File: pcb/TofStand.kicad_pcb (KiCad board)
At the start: 2 copper layers, 87 x 88 mm, 187 parts, among them Q1 BC848, Q10 BC848, Q11 BC848, Q14 MMBT2222, Q2 BC848, Q5 DVIUC6-4SC6, Q6 BC848, Q7 BC848, SW1 DIPx4, SW2 SWITCH_H, SW3 BUTTON, SW4 SWITCH_2x, SW5 SWITCH_2x, U1 L6470, U2 L6470

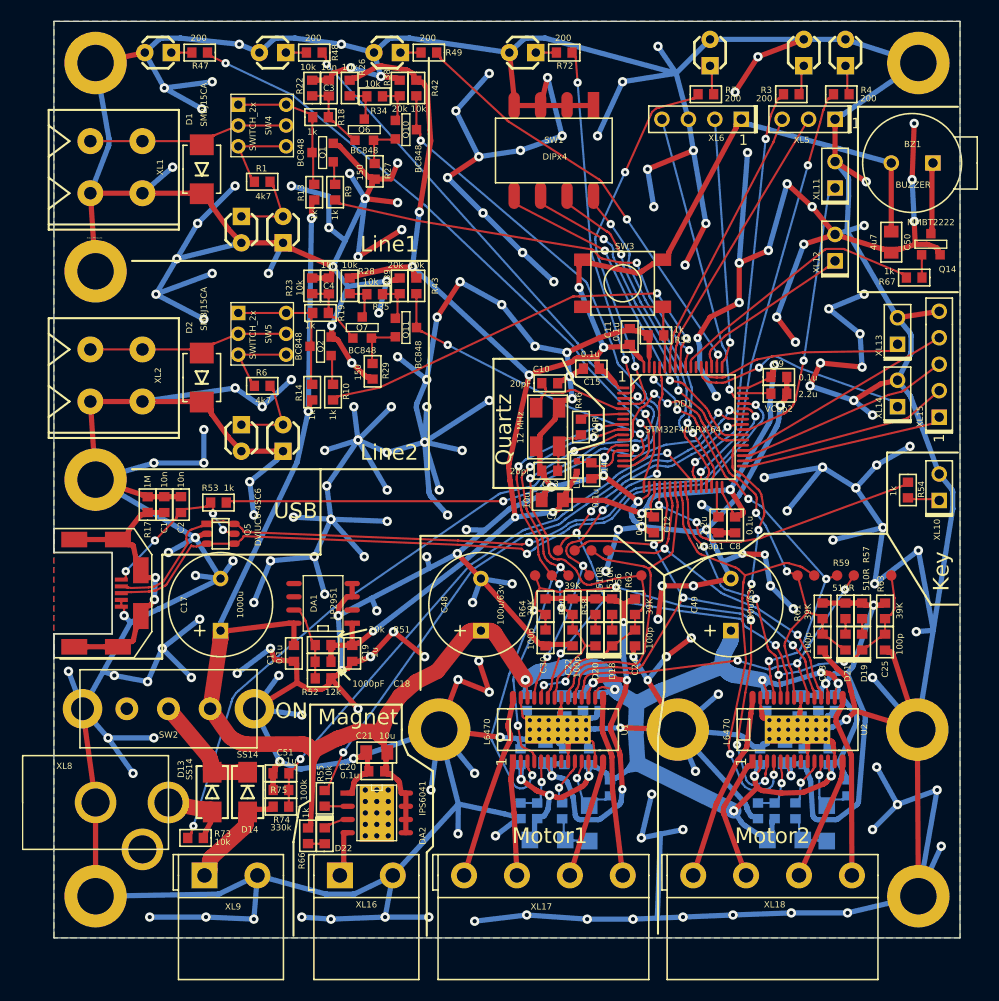
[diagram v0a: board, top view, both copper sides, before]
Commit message: PCB sent to factory
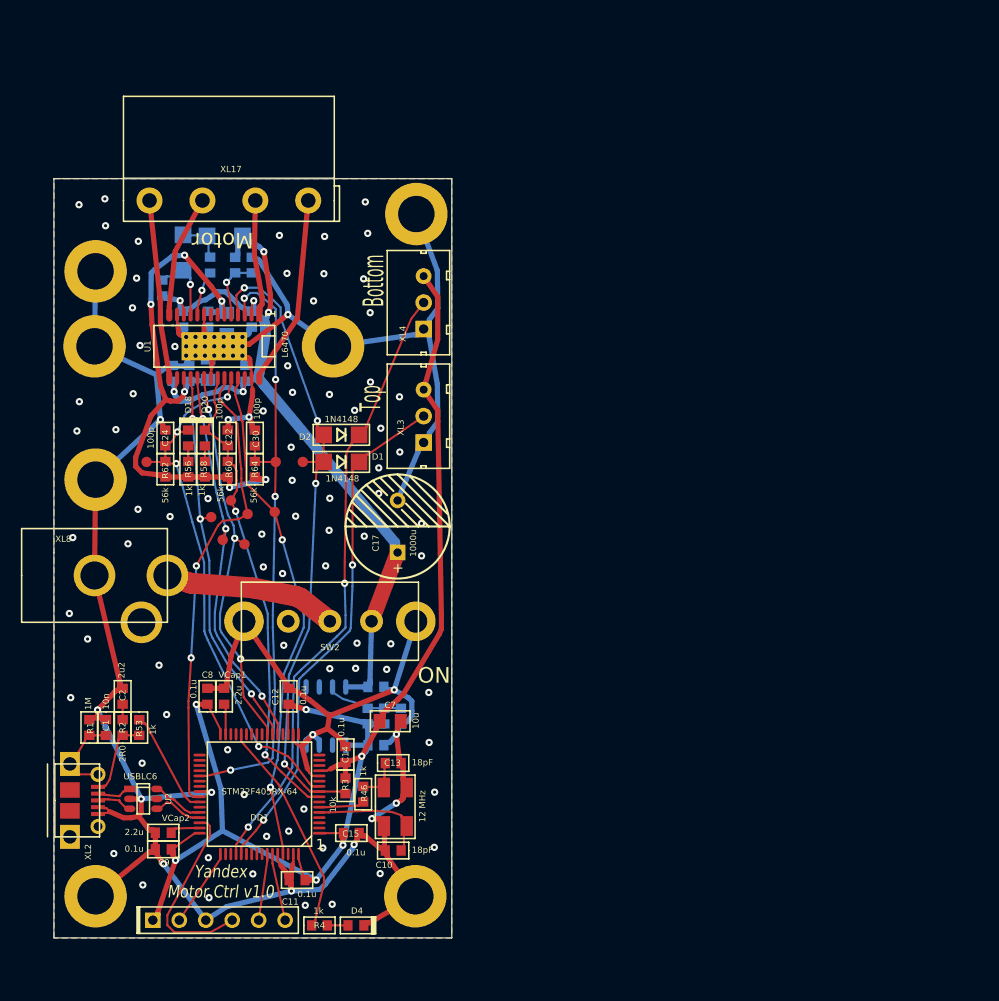
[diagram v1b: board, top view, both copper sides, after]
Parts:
- removed BZ1: BUZZER, Installation:BUZZER_HC0903
- removed C20, C28, C29, C51: 0.1u, Capacitors:CAP_0603
- removed C21, C34: 10u, Capacitors:CAP_0805
- removed C23, C25: 100p, Capacitors:CAP_0603
- removed C3, C4: 10n, Capacitors:CAP_0603
- removed C35: 4u7/63v, Capacitors:CAP_0805
- removed C38: 220n/16v, Capacitors:CAP_0603
- removed C39: 10n/50v, Capacitors:CAP_0603
- removed C41, C43, C45, C47: 0.1u/50v, Capacitors:CAP_0603
- removed C48, C49: 100u/63v, Capacitors:CAP_10xxR
- removed C50: 4u7, Capacitors:CAP_0805
- removed D10, D15, D16, D17, D27, D3, D5, D6, D7, D9: LED, LEDs:LED_Through-Hole-3mm
- removed D13, D14: SS14, Diodes:SMA_DO214AC
- removed D19, D21, D22: LED, LEDs:LED_0603
- removed D24, D26: 1N4148, Diodes:SOD80C
- removed DA2: IPS6041, SO_DIL_TSSOP:SO8HEATSINK
- removed HOLE3, HOLE9: HOLE_METALLED, PCB:Hole3_5_out6mm
- removed L1: BLM, Inductors:IND_0402
- removed Q1, Q10, Q11, Q2, Q6, Q7: BC848, SOT:SOT23-3
- removed Q14: MMBT2222, SOT:SOT23-3
- removed Q5: DVIUC6-4SC6, SOT:SOT23-6
- removed R10, R13, R14, R18, R19, R50, R54, R66, R67, R9: 1k, Resistors:RES_0603
- removed R17: 1M, Resistors:RES_0603
- removed R22, R23, R26, R28, R34, R35, R42, R43, R55, R73: 10k, Resistors:RES_0603
- removed R27, R29: 150, Resistors:RES_0603
- removed R38, R39: 20k, Resistors:RES_0603
- removed R47, R48, R49, R7, R72: 200, Resistors:RES_0603
- removed R57, R59: 510R, Resistors:RES_0603
- removed R6, R71: 4k7, Resistors:RES_0603
- removed R61, R63: 39K, Resistors:RES_0603
- removed R70: 33k, Resistors:RES_0603
- removed R74: 330k, Resistors:RES_0603
- removed R75: 100k, Resistors:RES_0603
- removed SW1: DIPx4, BtnsSwitches:DIP_SMD_X4
- removed SW3: BUTTON, BtnsSwitches:BTN_6x6
- removed SW4, SW5: SWITCH_2x, BtnsSwitches:BTN_PSM6
- removed TP10, TP11, TP12, TP13, TP14: TESTPOINT, PCB:TESTPOINT_1MM
- removed XL10, XL11, XL12, XL13, XL14: CONN_2, Connectors:PLS-2
- removed XL15: CONN_5, Connectors:PLS-5
- removed XL16, XL9: CONN_2, Connectors:TermiBlockHeader_508_x2_R
- removed XL18: CONN_4, Connectors:TermiBlockHeader_508_x4_R
- removed XL5: CONN_3, Connectors:PLS-3
- removed XL6: ST_SWD, Connectors:PLS-4
- removed XL7: USB_MICRO_B, Connectors:USBmicro_MOLEX_WM17142
- added R2: 2R0, Resistors:RES_0603, F.Cu at (74.6, 95.8)
- added XL3: CONN_3, Connectors:W03_Pitch_2d54, F.Cu at (103.5, 65.9)
- added XL4: CONN_3, Connectors:W03_Pitch_2d54, F.Cu at (103.5, 55.0)
- C10, C13: value 20pF -> 18pF
- C16, C18, C19, R51, R52: moved to B.Cu
- C2: value 10n -> 2u2
- C33: value 4u7/63v -> 10u
- C36: value 220n/16v -> 220n
- C37: value 10n/50v -> 10n
- C40, C42, C44, C46: value 0.1u/50v -> 0.1u
- D1, D2: value SMBJ15CA -> 1N4148; footprint Diodes:SMB_DO214AA -> Diodes:SOD80C
- D4: footprint LEDs:LED_Through-Hole-3mm -> LEDs:LED_0603
- DA1: footprint SO_DIL_TSSOP:SO8 -> SO_DIL_TSSOP:SO8_150MIL; moved to B.Cu
- R1: value 4k7 -> 1M
- R3: value 200 -> 10k
- R4: value 200 -> 1k
- R46: value 200R -> 1k
- R56, R58: value 510R -> 1k
- R60, R62, R64: value 39K -> 56k
- U2: value L6470 -> USBLC6; footprint SO_DIL_TSSOP:HTSSOP28 -> SOT:SOT23-6
- XL1: value CONN_2 -> CONN_6; footprint Connectors:SPRING_TERM_XY124V_A_2 -> Connectors:PLS-6
- XL2: value CONN_2 -> USB_MICRO; footprint Connectors:SPRING_TERM_XY124V_A_2 -> Connectors:USBmicro_MOLEX_1050170001
- moved D4 96.1 mm to (97.0, 114.8), turned to 0 degrees
- moved R4 94.2 mm to (93.5, 114.8)
- moved R3 79.0 mm to (96.0, 101.4), turned to 270 degrees
- moved C9 74.5 mm to (78.5, 107.5), turned to 180 degrees
- moved VCap2 72.6 mm to (78.5, 105.9), turned to 180 degrees
- moved XL1 72.4 mm to (77.5, 114.3), turned to 0 degrees
- moved XL17 71.5 mm to (84.8, 45.2), turned to 180 degrees
- moved D23 67.3 mm to (80.4, 50.2), turned to 90 degrees
- moved HOLE10 67.0 mm to (71.9, 59.2), turned to 180 degrees
- moved D25 65.8 mm to (84.4, 48.6), turned to 0 degrees
- moved C36 64.4 mm to (78.4, 53.6), turned to 270 degrees
- moved U2 63.2 mm to (76.6, 102.6)
- moved C37 62.4 mm to (83.0, 51.4), turned to 270 degrees
- moved TP6 62.1 mm to (86.6, 75.3)
- moved TP9 62.0 mm to (83.1, 75.6)
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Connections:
- net /LED_BT_LOW renamed Net-(DD1-Pad28)
- C1 pad 1: /SHLD -> GND
- C1 pad 2: GND -> Net-(C1-Pad2)
- C11 pad 1: +3.3V -> +3v3
- C12 pad 1: +3.3V -> +3v3
- C14 pad 1: Net-(C14-Pad1) -> +3v3
- C15 pad 1: +3.3V -> +3v3
- C16 pad 1: +12V -> +12v
- C17 pad 1: +12V -> +12v
- C18 pad 1: +3.3V -> +3v3
- C19 pad 1: +3.3V -> +3v3
- C2 pad 1: GND -> Net-(C2-Pad1)
- C2 pad 2: /5V_USB -> GND
- C36 pad 2: +12V -> +12v
- C40 pad 1: +12V -> +12v
- C42 pad 1: +12V -> +12v
- C44 pad 1: +12V -> +12v
- C46 pad 1: +12V -> +12v
- C7 pad 1: +3.3V -> +3v3
- C8 pad 1: +3.3V -> +3v3
- C9 pad 1: +3.3V -> +3v3
- D1 pad A: /LineIn1 -> /SW_1
- D1 pad C: GND -> /ENDSTOP_TOP
- D2 pad A: /LineIn2 -> /SW_1
- D2 pad C: GND -> /ENDSTOP_BOT
- D25 pad A: +12V -> +12v
- DA1 pad 1: +3.3V -> +3v3
- DA1 pad 8: +12V -> +12v
- DD1 pad 1: +3.3V -> +3v3
- DD1 pad 11: /BUSY/SYNC_2 -> (no net)
- DD1 pad 13: Net-(C14-Pad1) -> +3v3
- DD1 pad 14: /TrgOut1 -> (no net)
- DD1 pad 15: /TrgOut2 -> (no net)
- DD1 pad 16: /LED1 -> (no net)
- DD1 pad 17: /LED2 -> (no net)
- DD1 pad 19: +3.3V -> +3v3
- DD1 pad 2: /LED4 -> (no net)
- DD1 pad 20: Net-(DD1-Pad20) -> (no net)
- DD1 pad 24: /SW_2 -> (no net)
- DD1 pad 25: /FLAG_2 -> (no net)
- DD1 pad 26: /BatteryMeas -> (no net)
- DD1 pad 27: /LED_BT_PWR -> (no net)
- DD1 pad 29: /DS1 -> (no net)
- DD1 pad 3: /PwrSrcSns -> (no net)
- DD1 pad 30: /DS2 -> (no net)
- DD1 pad 32: +3.3V -> +3v3
- DD1 pad 33: /RSL1 -> (no net)
- DD1 pad 34: /RSL2 -> (no net)
- DD1 pad 35: /RSL3 -> (no net)
- DD1 pad 36: /RSL4 -> (no net)
- DD1 pad 38: /DS3 -> (no net)
- DD1 pad 39: /DS4 -> (no net)
- DD1 pad 4: /LED_SRC_PWR -> (no net)
- DD1 pad 40: /GPIO1 -> GND
- DD1 pad 43: /MagnetIN -> (no net)
- DD1 pad 44: /D- -> /USB_D-
- DD1 pad 45: /D+ -> /USB_D+
- DD1 pad 48: +3.3V -> +3v3
- DD1 pad 50: /LED3 -> (no net)
- DD1 pad 51: /GPIO2 -> (no net)
- DD1 pad 52: /GPIO3 -> /ENDSTOP_BOT
- DD1 pad 53: /GPIO4 -> /ENDSTOP_TOP
- DD1 pad 55: /Buzzer -> (no net)
- DD1 pad 56: /LineTx1 -> (no net)
- DD1 pad 57: /LineTx2 -> (no net)
- DD1 pad 58: /DBG_UART_TX -> /UART_TX
- DD1 pad 59: /DBG_UART_RX -> /UART_RX
- DD1 pad 60: Net-(DD1-Pad60) -> GND
- DD1 pad 62: /STEP_CLK_2 -> (no net)
- DD1 pad 64: +3.3V -> +3v3
- R1 pad 1: Net-(R1-Pad1) -> Net-(C1-Pad2)
- R1 pad 2: Net-(D5-PadA) -> GND
- R3 pad 1: /LED_BT_PWR -> +3v3
- R3 pad 2: Net-(D3-PadA) -> /SW_1
- R51 pad 1: +3.3V -> +3v3
- R68 pad 1: +12V -> +12v
- SW2 pad 1: +12V -> +12v
- TP4 pad 1: /BUSY/SYNC_2 -> /STEP_CLK_1
- TP5 pad 1: /SW_2 -> /STBY/RST
- TP6 pad 1: /FLAG_2 -> /MOTOR_CS
- TP7 pad 1: /STEP_CLK_1 -> /MOTOR_SCK
- TP8 pad 1: /STEP_CLK_2 -> /MOTOR_MOSI
- TP9 pad 1: /SDI_2 -> /MOTOR_MISO
- U1 pad 12: +12V -> +12v
- U1 pad 16: +12V -> +12v
- U1 pad 18: /SDI_2 -> /MOTOR_MISO
- U1 pad 2: +12V -> +12v
- U1 pad 26: +12V -> +12v
- U2 pad 1: /OUT2_1A -> /DIN-
- U2 pad 2: +12V -> GND
- U2 pad 3: /STBY/RST -> /DIN+
- U2 pad 4: /SW_2 -> /USB_D+
- U2 pad 5: /ADC_2 -> (no net)
- U2 pad 6: /Vdd2 -> /USB_D-
- XL1 pad 1: /LineIn1 -> +3v3
- XL1 pad 2: GND -> /SWCLK
- XL2 pad 1: /LineIn2 -> /5V_USB
- XL2 pad 2: GND -> /DIN-
- XL8 pad PWR: /PWR_SRC -> /PWR_IN
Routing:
- net GND: track 1506.7 -> 301.8 mm, vias 210 -> 94
- net +12V: track 251.9 -> 0.00 mm, vias 13 -> 0
- net +3.3V: track 215.7 -> 0.00 mm, vias 11 -> 0
- net +3v3: track 0.00 -> 136.9 mm, vias 0 -> 6
- net +12v: track 0.00 -> 86.7 mm, vias 0 -> 6
- net /D+: track 72.2 -> 0.00 mm, vias 2 -> 0
- net /D-: track 71.1 -> 0.00 mm, vias 2 -> 0
- net /PwrSrcSns: track 68.3 -> 0.00 mm, vias 2 -> 0
- net /LED1: track 61.3 -> 0.00 mm, vias 2 -> 0
- net /ENDSTOP_BOT: track 0.00 -> 58.8 mm, vias 0 -> 2
- net /MagnetIN: track 56.7 -> 0.00 mm, vias 2 -> 0
- net /BatteryMeas: track 55.9 -> 0.00 mm, vias 2 -> 0
- net /LED2: track 54.1 -> 0.00 mm, vias 2 -> 0
- net /ENDSTOP_TOP: track 0.00 -> 49.4 mm, vias 0 -> 2
- net /BUSY/SYNC_2: track 48.4 -> 0.00 mm, vias 4 -> 0
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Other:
- board size 87 x 88 mm -> 38.2 x 72.9 mm
- net class Default: via_dia 0.8 -> 0.7
- net class Wide: via_dia 0.9 -> 0.7; via_drill 0.4 -> 0.3
- rule pad_to_mask_clearance: 0.1 -> 0.06
- rule solder_mask_min_width: 0.2 -> 0.15
- board text added: "Bottom"
- board text added: "Motor"
- board text added: "Top"
- board text added: "Yandex Motor Ctrl v1.0"
- board text removed: "Key"
- board text removed: "Line1"
- board text removed: "Line2"
- board text removed: "Magnet"
- board text removed: "Motor1"
- board text removed: "Motor2"
- board text removed: "Quartz"
- board text removed: "USB"
